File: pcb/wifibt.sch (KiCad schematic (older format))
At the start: 15 parts, among them Q800 IRLML6402, U800 RTL8723BS

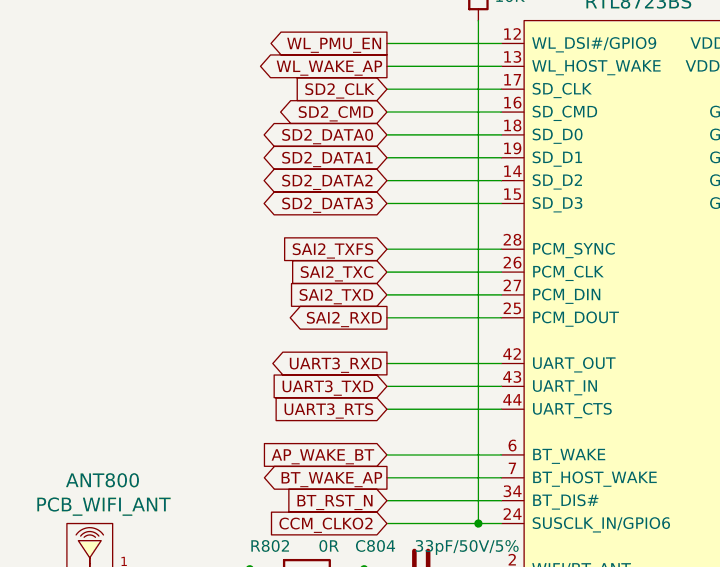
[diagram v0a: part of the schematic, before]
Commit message: pcb: finishing sch for r0.1
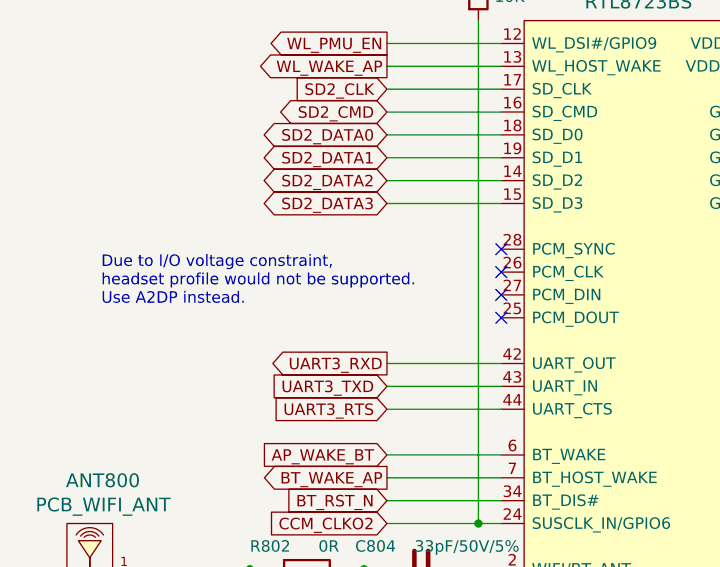
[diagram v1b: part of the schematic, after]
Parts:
- C800, C802, C804, C805, C806: footprint (none) -> Capacitor_SMD:C_0402_1005Metric
- C801, C803: footprint (none) -> Capacitor_SMD:C_0603_1608Metric
- D800: footprint (none) -> Diode_SMD:D_SOD-523
- R800, R801, R802, R803: footprint (none) -> Resistor_SMD:R_0603_1608Metric
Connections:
- net SAI2_RXD: no longer names the net of U800.25 (PCM_DOUT)
- net SAI2_TXC: no longer names the net of U800.26 (PCM_CLK)
- net SAI2_TXD: no longer names the net of U800.27 (PCM_DIN)
- net SAI2_TXFS: no longer names the net of U800.28 (PCM_SYNC)
- no-connect marks 0 -> 4
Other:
- note added: "Due to I/O voltage constraint,\nheadset profile would not be supported.\nUse A2DP instead."
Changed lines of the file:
@@
 F 0 "C800" H 6815 3496 50  0000 L CNN
 F 1 "100nF" H 6815 3405 50  0000 L CNN
-F 2 "" H 6738 3300 50  0001 C CNN
+F 2 "Capacitor_SMD:C_0402_1005Metric" H 6738 3300 50  0001 C CNN
 F 3 "~" H 6700 3450 50  0001 C CNN
 	1    6700 3450
@@
 F 0 "C801" H 7315 3496 50  0000 L CNN
 F 1 "10uF" H 7315 3405 50  0000 L CNN
-F 2 "" H 7238 3300 50  0001 C CNN
+F 2 "Capacitor_SMD:C_0603_1608Metric" H 7238 3300 50  0001 C CNN
 F 3 "~" H 7200 3450 50  0001 C CNN
 	1    7200 3450
@@
 F 0 "C802" H 7815 3496 50  0000 L CNN
 F 1 "100nF" H 7815 3405 50  0000 L CNN
-F 2 "" H 7738 3300 50  0001 C CNN
+F 2 "Capacitor_SMD:C_0402_1005Metric" H 7738 3300 50  0001 C CNN
 F 3 "~" H 7700 3450 50  0001 C CNN
 	1    7700 3450
@@
 F 0 "C803" H 8315 3496 50  0000 L CNN
 F 1 "10uF" H 8315 3405 50  0000 L CNN
-F 2 "" H 8238 3300 50  0001 C CNN
+F 2 "Capacitor_SMD:C_0603_1608Metric" H 8238 3300 50  0001 C CNN
 F 3 "~" H 8200 3450 50  0001 C CNN
 	1    8200 3450
@@
 $EndComp
 $Comp
-L power:GND #PWR?
+L power:GND #PWR0306
 U 1 1 5D1C6F63
 P 7700 3700
-F 0 "#PWR?" H 7700 3450 50  0001 C CNN
+F 0 "#PWR0306" H 7700 3450 50  0001 C CNN
 F 1 "GND" H 7705 3527 50  0000 C CNN
 F 2 "" H 7700 3700 50  0001 C CNN
@@
 AR Path="/5DB2122B/5D1E0260" Ref="#PWR?"  Part="1"
 AR Path="/5DB51F59/5D1E0260" Ref="#PWR?"  Part="1"
-AR Path="/5D1BA41C/5D1E0260" Ref="#PWR?"  Part="1"
-F 0 "#PWR?" H 6700 1750 50  0001 C CNN
+AR Path="/5D1BA41C/5D1E0260" Ref="#PWR0307"  Part="1"
+F 0 "#PWR0307" H 6700 1750 50  0001 C CNN
 F 1 "+3V3" H 6715 2073 50  0000 C CNN
 F 2 "" H 6700 1900 50  0001 C CNN
@@
 F 0 "R801" H 6270 2496 50  0000 L CNN
 F 1 "10K" H 6270 2405 50  0000 L CNN
-F 2 "" V 6130 2450 50  0001 C CNN
+F 2 "Resistor_SMD:R_0603_1608Metric" V 6130 2450 50  0001 C CNN
 F 3 "~" H 6200 2450 50  0001 C CNN
 	1    6200 2450
@@
 F 0 "R800" H 6270 1996 50  0000 L CNN
 F 1 "100K" H 6270 1905 50  0000 L CNN
-F 2 "" V 6130 1950 50  0001 C CNN
+F 2 "Resistor_SMD:R_0603_1608Metric" V 6130 1950 50  0001 C CNN
 F 3 "~" H 6200 1950 50  0001 C CNN
 	1    6200 1950
@@
 AR Path="/5DB2122B/5D1E027E" Ref="#PWR?"  Part="1"
 AR Path="/5DB51F59/5D1E027E" Ref="#PWR?"  Part="1"
-AR Path="/5D1BA41C/5D1E027E" Ref="#PWR?"  Part="1"
-F 0 "#PWR?" H 6200 2350 50  0001 C CNN
+AR Path="/5D1BA41C/5D1E027E" Ref="#PWR0308"  Part="1"
+F 0 "#PWR0308" H 6200 2350 50  0001 C CNN
 F 1 "GND" H 6205 2427 50  0000 C CNN
 F 2 "" H 6200 2600 50  0001 C CNN
@@
 AR Path="/5DB2122B/5D1E0284" Ref="#PWR?"  Part="1"
 AR Path="/5DB51F59/5D1E0284" Ref="#PWR?"  Part="1"
-AR Path="/5D1BA41C/5D1E0284" Ref="#PWR?"  Part="1"
-F 0 "#PWR?" H 6200 1650 50  0001 C CNN
+AR Path="/5D1BA41C/5D1E0284" Ref="#PWR0309"  Part="1"
+F 0 "#PWR0309" H 6200 1650 50  0001 C CNN
 F 1 "+3V3" H 6215 1973 50  0000 C CNN
 F 2 "" H 6200 1800 50  0001 C CNN
@@
 F 0 "D800" H 5950 1984 50  0000 C CNN
 F 1 "RB521S30T1G" H 5950 2075 50  0000 C CNN
-F 2 "" H 5950 2200 50  0001 C CNN
+F 2 "Diode_SMD:D_SOD-523" H 5950 2200 50  0001 C CNN
 F 3 "~" H 5950 2200 50  0001 C CNN
 	1    5950 2200
@@
 Connection ~ 7700 3600
 $Comp
-L power:GND #PWR?
+L power:GND #PWR0310
 U 1 1 5D1C677C
 P 6700 3700
-F 0 "#PWR?" H 6700 3450 50  0001 C CNN
+F 0 "#PWR0310" H 6700 3450 50  0001 C CNN
 F 1 "GND" H 6705 3527 50  0000 C CNN
 F 2 "" H 6700 3700 50  0001 C CNN
@@
 $EndComp
 $Comp
-L power:GND #PWR?
+L power:GND #PWR0311
 U 1 1 5D1E38E1
 P 6500 3900
-F 0 "#PWR?" H 6500 3650 50  0001 C CNN
+F 0 "#PWR0311" H 6500 3650 50  0001 C CNN
 F 1 "GND" H 6505 3727 50  0000 C CNN
 F 2 "" H 6500 3900 50  0001 C CNN
@@
 F 0 "C804" V 4750 5200 50  0000 C CNN
 F 1 "33pF/50V/5%" V 4750 5600 50  0000 C CNN
-F 2 "" H 4888 5250 50  0001 C CNN
+F 2 "Capacitor_SMD:C_0402_1005Metric" H 4888 5250 50  0001 C CNN
 F 3 "~" H 4850 5400 50  0001 C CNN
 	1    4850 5400
@@
 F 0 "C805" H 4485 5604 50  0000 R CNN
 F 1 "DNP" H 4485 5695 50  0000 R CNN
-F 2 "" H 4638 5500 50  0001 C CNN
+F 2 "Capacitor_SMD:C_0402_1005Metric" H 4638 5500 50  0001 C CNN
 F 3 "~" H 4600 5650 50  0001 C CNN
 	1    4600 5650
@@
 F 0 "R802" V 4250 5150 50  0000 L CNN
 F 1 "0R" V 4250 5450 50  0000 L CNN
-F 2 "" V 4280 5400 50  0001 C CNN
+F 2 "Resistor_SMD:R_0603_1608Metric" V 4280 5400 50  0001 C CNN
 F 3 "~" H 4350 5400 50  0001 C CNN
 	1    4350 5400
@@
 F 0 "C806" H 3985 5604 50  0000 R CNN
 F 1 "DNP" H 3985 5695 50  0000 R CNN
-F 2 "" H 4138 5500 50  0001 C CNN
+F 2 "Capacitor_SMD:C_0402_1005Metric" H 4138 5500 50  0001 C CNN
 F 3 "~" H 4100 5650 50  0001 C CNN
 	1    4100 5650
@@
 $EndComp
 $Comp
-L power:GND #PWR?
+L power:GND #PWR0312
 U 1 1 5D1EA804
 P 3700 5600
-F 0 "#PWR?" H 3700 5350 50  0001 C CNN
+F 0 "#PWR0312" H 3700 5350 50  0001 C CNN
 F 1 "GND" H 3705 5427 50  0000 C CNN
 F 2 "" H 3700 5600 50  0001 C CNN
@@
 $EndComp
 $Comp
-L power:GND #PWR?
+L power:GND #PWR0313
 U 1 1 5D1EAE49
 P 4100 5900
-F 0 "#PWR?" H 4100 5650 50  0001 C CNN
+F 0 "#PWR0313" H 4100 5650 50  0001 C CNN
 F 1 "GND" H 4105 5727 50  0000 C CNN
 F 2 "" H 4100 5900 50  0001 C CNN
@@
 $EndComp
 $Comp
-L power:GND #PWR?
+L power:GND #PWR0314
 U 1 1 5D1EB029
 P 4600 5900
-F 0 "#PWR?" H 4600 5650 50  0001 C CNN
+F 0 "#PWR0314" H 4600 5650 50  0001 C CNN
 F 1 "GND" H 4605 5727 50  0000 C CNN
 F 2 "" H 4600 5900 50  0001 C CNN
@@
 $EndComp
 $Comp
-L power:GND #PWR?
+L power:GND #PWR0315
 U 1 1 5D1EB239
 P 5100 5600
-F 0 "#PWR?" H 5100 5350 50  0001 C CNN
+F 0 "#PWR0315" H 5100 5350 50  0001 C CNN
 F 1 "GND" H 5105 5427 50  0000 C CNN
 F 2 "" H 5100 5600 50  0001 C CNN
@@
 Text GLabel 4700 4900 0    50   Input ~ 0
 AP_WAKE_BT
-Text GLabel 4700 4300 0    50   Output ~ 0
-SAI2_RXD
-Text GLabel 4700 4200 0    50   Input ~ 0
-SAI2_TXD
-Text GLabel 4700 4100 0    50   Input ~ 0
-SAI2_TXC
-Text GLabel 4700 4000 0    50   Input ~ 0
-SAI2_TXFS
 Text GLabel 4700 4500 0    50   Output ~ 0
 UART3_RXD
@@
 Text GLabel 4700 4700 0    50   Input ~ 0
 UART3_RTS
-Wire Wire Line
-	4700 4000 5200 4000
-Wire Wire Line
-	4700 4100 5200 4100
-Wire Wire Line
-	4700 4200 5200 4200
-Wire Wire Line
-	4700 4300 5200 4300
 Wire Wire Line
 	4700 4500 5200 4500
@@
 F 0 "R803" H 5170 2896 50  0000 L CNN
 F 1 "10K" H 5170 2805 50  0000 L CNN
-F 2 "" V 5030 2850 50  0001 C CNN
+F 2 "Resistor_SMD:R_0603_1608Metric" V 5030 2850 50  0001 C CNN
 F 3 "~" H 5100 2850 50  0001 C CNN
 	1    5100 2850
@@
 	4700 5200 5100 5200
 Connection ~ 5100 5200
+NoConn ~ 5200 4000
+NoConn ~ 5200 4100
+NoConn ~ 5200 4200
+NoConn ~ 5200 4300
+Text Notes 3450 4250 0    50   ~ 0
+Due to I/O voltage constraint,\nheadset profile would not be supported.\nUse A2DP instead.
 $EndSCHEMATC
